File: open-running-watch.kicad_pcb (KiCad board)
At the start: 4 copper layers, 41 x 61.9 mm, 211 parts, among them IC1 BLUENRG-232N, IC10 NXB0108BQX, IC11 STM32L475RGT6, IC12 W25N512GVEIG, IC13 TPS613222ADBVR, IC14 INA186A5IYFDR, IC15 INA186A5IYFDR, IC16 INA186A5IYFDR, IC17 INA186A5IYFDR, IC18 PCAL9538ABSHP, IC19 INA186A5IYFDR, IC2 TESEO-LIV3F, IC20 INA186A5IYFDR, IC21 LSF0204GU12X, IC22 INA186A5IYFDR, IC3 BGA_725L6_E6327, IC4 BQ27441DRZR-G1A, IC5 MCP73811T-420I_OT, IC6 TPS62237DRYR, IC7 ST1S15J18R, IC8 TLV9002SIRUGR, IC9 ICP-10100, J1 20021121-00014T4LF, J2 10118192-0001LF, J3 1-2328702-0, J4 2328702-4, Q1 BC847BS, Q2 BC847BS, Q3 PMN280ENEAX, Q4 BC846, Q5 BC846, T1 BALF-NRG-02D3, U1 TPS62233DRYR, Y1 ECS-320-12-37B2-7KM-TR, Y2 NX3215SA-32.768K-EXS00A-MU000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, Y3 ECS-.327-7-1210-TR

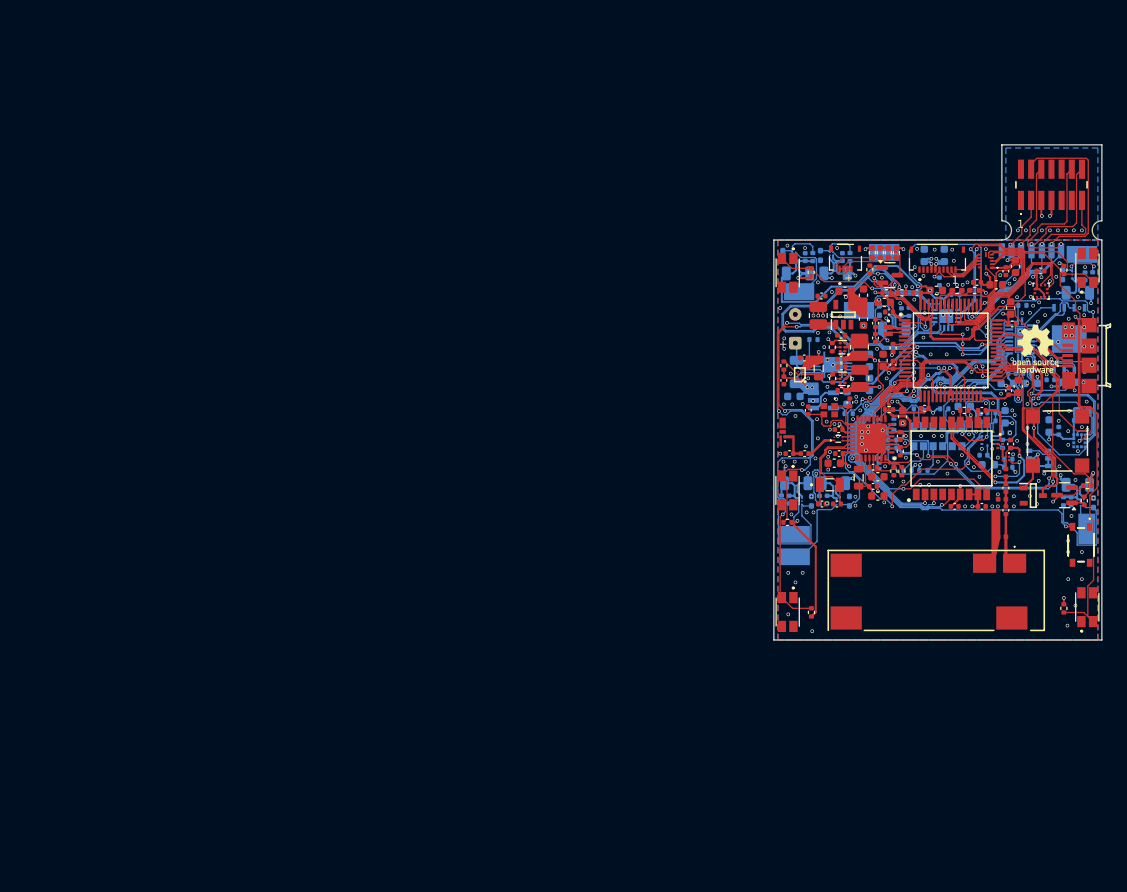
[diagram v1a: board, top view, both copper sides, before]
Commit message: TEMP COMMIT
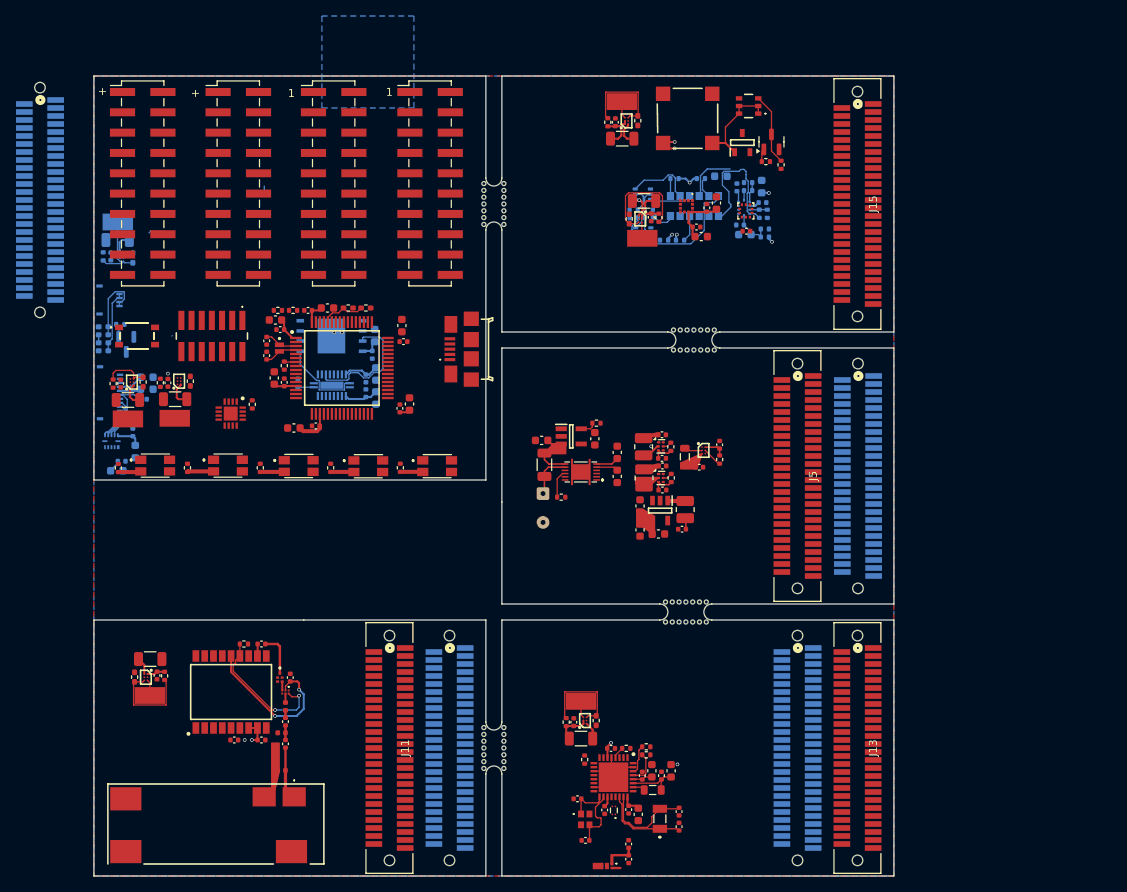
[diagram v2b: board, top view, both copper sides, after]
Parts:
- removed G***: LOGO, pcbway-logo:pcbway-logo
- removed LOGO1: OSHW-Logo_5.7x6mm_SilkScreen, Symbol:OSHW-Logo_5.7x6mm_SilkScreen
- added J10: Conn_02x10_Odd_Even, Connector_PinHeader_2.54mm:PinHeader_2x10_P2.54mm_Vertical_SMD, F.Cu at (86.5, 66.9)
- added J11: DF9-51P-1V69, DF9-51P-1V(69):CON9_1X51_MDZL_DF9_HIR, F.Cu at (81.4, 137.5)
- added J12: DF9-51S-1V69, DF9-51S-1V(69):CON9_1X51_DZL_DF9_HIR, B.Cu at (88.9, 137.5)
- added J13: DF9-51P-1V69, DF9-51P-1V(69):CON9_1X51_MDZL_DF9_HIR, F.Cu at (139.9, 137.5)
- added J14: DF9-51S-1V69, DF9-51S-1V(69):CON9_1X51_DZL_DF9_HIR, B.Cu at (132.4, 137.5)
- added J15: DF9-51P-1V69, DF9-51P-1V(69):CON9_1X51_MDZL_DF9_HIR, F.Cu at (139.9, 69.5)
- added J18: DF9-51S-1V69, DF9-51S-1V(69):CON9_1X51_DZL_DF9_HIR, B.Cu at (37.8, 69.0)
- added J5: DF9-51P-1V69, DF9-51P-1V(69):CON9_1X51_MDZL_DF9_HIR, F.Cu at (132.4, 103.5)
- added J6: DF9-51S-1V69, DF9-51S-1V(69):CON9_1X51_DZL_DF9_HIR, B.Cu at (140.0, 103.5)
- added J7: Conn_02x10_Odd_Even, Connector_PinHeader_2.54mm:PinHeader_2x10_P2.54mm_Vertical_SMD, F.Cu at (50.6, 66.9)
- added J8: Conn_02x10_Odd_Even, Connector_PinHeader_2.54mm:PinHeader_2x10_P2.54mm_Vertical_SMD, F.Cu at (62.6, 66.9)
- added J9: Conn_02x10_Odd_Even, Connector_PinHeader_2.54mm:PinHeader_2x10_P2.54mm_Vertical_SMD, F.Cu at (74.5, 66.9)
- added REF**: MouseBite-Slot_2.0x4.5mm_inset_D0.5mm_P0.85mm_7h, Panelization:MouseBite-Slot_2.0x4.5mm_inset_D0.5mm_P0.85mm_7h, F.Cu at (119.5, 85.5)
- added REF**: MouseBite-Slot_2.0x4.5mm_inset_D0.5mm_P0.85mm_7h, Panelization:MouseBite-Slot_2.0x4.5mm_inset_D0.5mm_P0.85mm_7h, F.Cu at (118.5, 119.5)
- added REF**: MouseBite-Slot_2.0x4.5mm_inset_D0.5mm_P0.85mm_7h, Panelization:MouseBite-Slot_2.0x4.5mm_inset_D0.5mm_P0.85mm_7h, F.Cu at (93.5, 69.5)
- added REF**: MouseBite-Slot_2.0x4.5mm_inset_D0.5mm_P0.85mm_7h, Panelization:MouseBite-Slot_2.0x4.5mm_inset_D0.5mm_P0.85mm_7h, F.Cu at (93.5, 137.5)
- AC1, BT1, C22, C23, C24, C25, C38, C39, C40, C41, C72, C73, C74, C75, C77, C78, IC14, IC15, IC16, IC17, IC18, IC19, IC20, IC4, IC5, Q3, R34, R35, R36, R37, R38, R39, R40, R41, R42, R43, R44, R45, R50, R51, R52, R53, R54, R55, R6, R65, R7, R8, TP1, TP2, TP3, TP4, TP6, TP7: moved to F.Cu
- C79, C80, C81, C82, IC21, J3, J4, Q4, R46, R59, R60, R61, R62: moved to B.Cu
- moved S1 120.9 mm to (49.9, 86.0), turned to 0 degrees
- moved R31 120.8 mm to (47.6, 102.5)
- moved S4 119.4 mm to (51.9, 102.2), turned to 0 degrees
- moved R35 117.3 mm to (52.8, 91.8)
- moved C72 115.4 mm to (53.8, 91.8)
- moved TP1 115.2 mm to (54.6, 96.3)
- moved C82 115.2 mm to (47.4, 102.8), turned to 180 degrees
- moved R34 113.6 mm to (54.7, 93.9), turned to 0 degrees
- moved C81 113.1 mm to (48.0, 101.6), turned to 180 degrees
- moved IC14 112.6 mm to (55.2, 91.7)
- moved IC21 111.6 mm to (46.7, 99.1), turned to 90 degrees
- moved R36 109.9 mm to (56.6, 91.7)
- moved C79 109.6 mm to (49.7, 100.4), turned to 90 degrees
- moved C80 107.2 mm to (49.4, 98.0), turned to -90 degrees
- moved J1 106.6 mm to (59.2, 86.0), turned to 180 degrees
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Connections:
- net /accelerometer/1V8 renamed /1V8
- net /audio/VCC_IN renamed /3V
- net /controller/OTG_FS_BUS renamed /VUSB
- net /mip_display/DISP_VDD renamed /5V
- net /power/3V3_EN renamed /PWR_3V3_EN
- net /power/3V_EN renamed /PWR_3V_EN
- AC1 pad 1: /accelerometer/SPC -> /SENS_SPC
- AC1 pad 11: /accelerometer/INT_2 -> /SENS_INT_2
- AC1 pad 12: /accelerometer/INT_1 -> /SENS_INT_1
- AC1 pad 2: /accelerometer/CS -> /SENS_CS
- AC1 pad 3: /accelerometer/SDO -> /SENS_SDO
- AC1 pad 4: /accelerometer/SDIO -> /SENS_SDIO
- C27 pad 1: /biometric/VCC_IN -> /3V3
- C52 pad 1: /biometric/VCC_IN -> /3V3_FLASH
- C57 pad 1: /biometric/VCC_IN -> /3V3_FLASH
- C72 pad 2: /biometric/VCC_IN -> /3V3_FLASH
- C78 pad 2: /biometric/VCC_IN -> /3V3
- IC1 pad 10: /accelerometer/SDO -> /BT_SPI_OUT
- IC1 pad 12: /accelerometer/SPC -> /BT_SPI_CLK
- IC1 pad 25: /bluenrg/RESET_N -> /BT_RESET_N
- IC1 pad 32: /bluenrg/SPI_CS -> /BT_SPI_CS
- IC1 pad 4: /bluenrg/SPI_IRQ -> /BT_SPI_IRQ
- IC1 pad 9: /accelerometer/SDIO -> /BT_SPI_IN
- IC11 pad 10: /biometric/OUT_IR_EN -> /MCU_HR_OUT_IR_EN
- IC11 pad 11: /bluenrg/RESET_N -> /MCU_BT_RESET_N
- IC11 pad 14: /bluenrg/SPI_IRQ -> /MCU_BT_IRQ
- IC11 pad 15: /bluenrg/SPI_CS -> /MCU_SPI_CS_2
- IC11 pad 16: /controller/USART2_TX -> /MCU_USART_TX
- IC11 pad 17: /controller/USART2_RX -> /MCU_USART_RX
- IC11 pad 20: /controller/GPS_RESET_N -> /MCU_GPS_RESET_N
- IC11 pad 24: /controller/GPS_WAKEUP -> /MCU_GPS_WAKEUP
- IC11 pad 25: /biometric/IN_G2 -> /MCU_HR_LED_G_2
- IC11 pad 28: /biometric/IN_IR -> /MCU_HR_LED_IR
- IC11 pad 33: /biometric/IN_R -> /MCU_HR_LED_R
- IC11 pad 34: /accelerometer/SPC -> /MCU_SPI_SCL
- IC11 pad 35: /accelerometer/SDO -> /MCU_SPI_MISO
- IC11 pad 36: /accelerometer/SDIO -> /MCU_SPI_MOSI
- IC11 pad 37: /accelerometer/CS -> /MCU_SPI_CS_1
- IC11 pad 38: /biometric/IN_G1 -> /MCU_HR_LED_G_1
- IC11 pad 39: /audio/IN -> /MCU_PWM
- IC11 pad 41: /accelerometer/INT_2 -> /MCU_ACC_IRQ_2
- IC11 pad 48: /biometric/VCC_IN -> /3V3_FLASH
- IC11 pad 59: /accelerometer/INT_1 -> /MCU_ACC_IRQ_1
- IC11 pad 61: /barometer/SCL -> /MCU_I2C_SCL
- IC11 pad 62: /barometer/SDA -> /MCU_I2C_SDA
- IC11 pad 8: /biometric/VOUT_RG -> /MCU_ADC_IN1
- IC11 pad 9: /biometric/VOUT_IR -> /MCU_ADC_IN2
- IC14 pad A1: /biometric/VCC_IN -> /3V3_FLASH
- IC14 pad A2: /biometric/VCC_IN -> /3V3_FLASH
- IC18 pad 12: /barometer/SCL -> /MCU_I2C_SCL
- IC18 pad 13: /barometer/SDA -> /MCU_I2C_SDA
- IC2 pad 2: /controller/USART2_RX -> /GPS_TX
- IC2 pad 3: /controller/USART2_TX -> /GPS_RX
- IC2 pad 4: /gps/PPS -> /GPS_PPS
- IC2 pad 5: /controller/GPS_WAKEUP -> /GPS_WAKEUP
- IC2 pad 9: /controller/GPS_RESET_N -> /GPS_RESET_N
- IC20 pad A1: /biometric/VCC_IN -> /3V3
- IC20 pad A2: /biometric/VCC_IN -> /3V3
- IC4 pad 1: /barometer/SDA -> /PWR_FUEL_SDA
- IC4 pad 12: /power/FUEL_LOW -> /PWR_FUEL_LOW
- IC4 pad 2: /barometer/SCL -> /PWR_FUEL_SCL
- IC6 pad 6: /biometric/VCC_IN -> /3V3
- IC8 pad 2: /biometric/OUT_IR_EN -> /SENS_OUT_RG_EN
- IC8 pad 3: /biometric/OUT_IR_EN -> /SENS_OUT_IR_EN
- IC8 pad 6: /biometric/VOUT_IR -> /SENS_VOUT_IR
- IC8 pad 8: /biometric/VOUT_RG -> /SENS_VOUT_RG
- IC9 pad 2: /barometer/SCL -> /SENS_SCL
- IC9 pad 4: /barometer/SDA -> /SENS_SDA
- L4 pad 1: /biometric/VCC_IN -> /3V3
- R1 pad 1: /bluenrg/SPI_IRQ -> /BT_SPI_IRQ
- R15 pad 2: /biometric/IN_G1 -> /SENS_IN_G1
- R17 pad 2: /biometric/IN_G2 -> /SENS_IN_G2
- R18 pad 2: /biometric/VOUT_IR -> /SENS_VOUT_IR
- R19 pad 1: /biometric/VOUT_IR -> /SENS_VOUT_IR
- R2 pad 1: /accelerometer/SDIO -> /BT_SPI_IN
- R20 pad 2: /biometric/IN_IR -> /SENS_IN_IR
- R21 pad 2: /biometric/VOUT_RG -> /SENS_VOUT_RG
- R24 pad 1: /biometric/VOUT_RG -> /SENS_VOUT_RG
- R25 pad 2: /biometric/IN_R -> /SENS_IN_R
- R27 pad 1: /barometer/SDA -> /MCU_I2C_SDA
- R28 pad 1: /barometer/SCL -> /MCU_I2C_SCL
- R34 pad 1: /biometric/VCC_IN -> /3V3_FLASH
- R35 pad 1: /biometric/VCC_IN -> /3V3_FLASH
- R53 pad 1: /biometric/VCC_IN -> /3V3
- R54 pad 1: /biometric/VCC_IN -> /3V3
- R64 pad 2: /audio/IN -> /SENS_IN
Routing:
- net /1V8: track 225.8 -> 15.2 mm, vias 13 -> 0
- net /controller/NRST: track 99.3 -> 1.40 mm, vias 3 -> 0
- net /barometer/SDA: track 87.1 -> 0.00 mm, vias 2 -> 0
- net /biometric/VCC_IN: track 77.5 -> 0.00 mm, vias 4 -> 0
- net /barometer/SCL: track 77.2 -> 0.00 mm, vias 1 -> 0
- net Net-(IC18-P1): track 73.5 -> 2.81 mm, vias 1 -> 0
- net Net-(IC18-P5): track 69.3 -> 2.91 mm, vias 3 -> 0
- net /3V: track 67.7 -> 5.45 mm, vias 3 -> 0
- net /accelerometer/INT_1: track 52.9 -> 0.00 mm, vias 6 -> 0
- net Net-(IC18-P4): track 54.0 -> 3.00 mm, vias 3 -> 0
- net /biometric/IN_G1: track 48.2 -> 0.00 mm, vias 3 -> 0
- net /controller/VDD: track 66.6 -> 20.3 mm, vias 9 -> 0
- net /biometric/OUT_IR_EN: track 46.0 -> 0.00 mm, vias 3 -> 0
- net /accelerometer/SDO: track 43.1 -> 0.00 mm, vias 1 -> 0
- net /accelerometer/SPC: track 42.8 -> 0.00 mm, vias 3 -> 0
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- removed copper zone on In2.Cu, net /5V
- removed copper zone on In2.Cu, net /audio/VCC
- removed copper zone on In2.Cu, net /biometric/VCC
- removed copper zone on In2.Cu, net /bluenrg/VBAT
- removed copper zone on In2.Cu, net /controller/VCC_FLASH
- removed copper zone on In2.Cu, net /controller/VDD
- removed copper zone on In2.Cu, net /gps/VCC
- removed copper zone on In2.Cu, net /mip_display/DISP_VDDIO
- removed copper zone on In2.Cu, net /power/SRN
- removed copper zone on In1.Cu, net GND
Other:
- board size 41 x 61.9 mm -> 100 x 100 mm
- board text removed: "1V8"
- board text removed: "GND"
- board text removed: "NRST"
- board text removed: "RX"
- board text removed: "SWCLK"
- board text removed: "SWDIO"
- board text removed: "Sponsored by"
- board text removed: "TX"
- board text removed: "github.com/fuad1502/open-running-watch-hw"
- board text removed: "v0.2.2"
